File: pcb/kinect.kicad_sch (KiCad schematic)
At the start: 22 parts, among them J2 USB_C_Receptacle_USB2.0_16P, J3 Conn_02x05_Odd_Even, U1 LM3670MFX-1.8, U2 AP63203WU

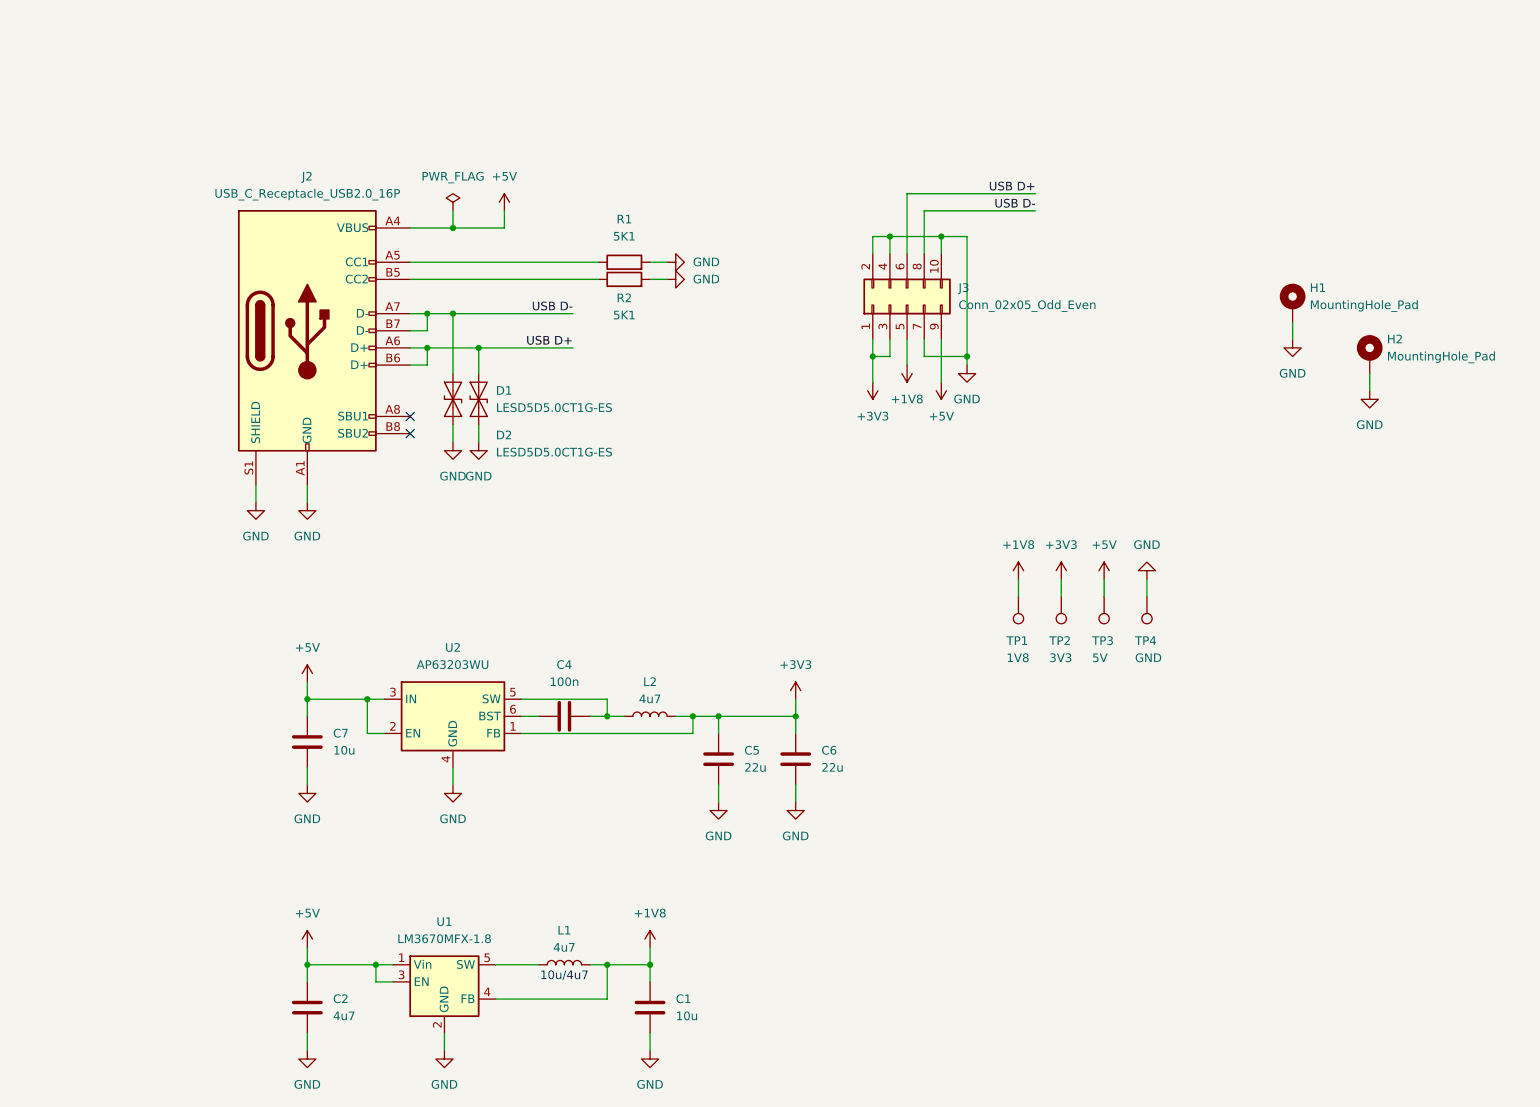
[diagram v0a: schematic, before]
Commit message: Beautified the design.
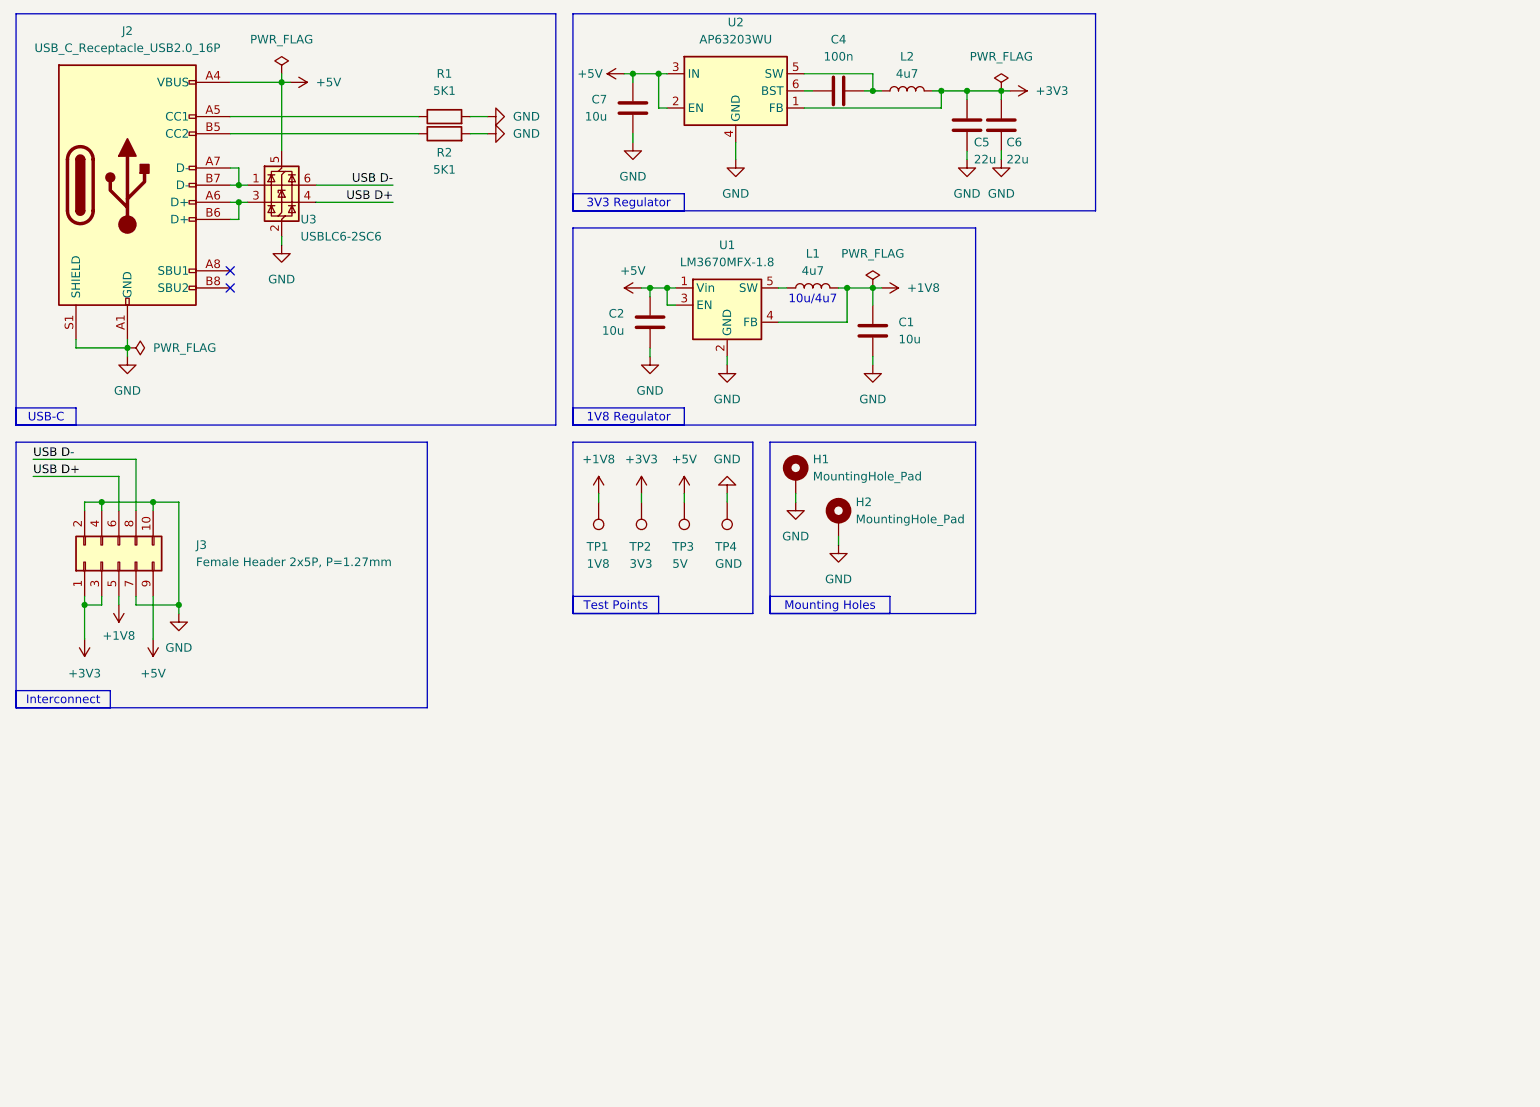
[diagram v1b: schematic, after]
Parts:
- removed D1, D2: LESD5D5.0CT1G-ES, Diode_SMD:D_SOD-523, symbol Diode:SMAJ440CA
- added U3: USBLC6-2SC6, Package_TO_SOT_SMD:SOT-23-6_Handsoldering, symbol Power_Protection:USBLC6-2SC6
- C2: value 4u7 -> 10u; LCSC C2918489 -> C1691
- C4: LCSC (none) -> C6119867
- J3: value Conn_02x05_Odd_Even -> Female Header 2x5P, P=1.27mm
- TP1, TP2, TP3, TP4: now left out of the parts list
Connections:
- net +5V: now also U3.5 (VBUS)
- net GND: now also U3.2 (GND)
- net USB D+: now also U3.4 (I/O2); no longer J2.A6 (D+), J2.B6 (D+)
- net USB D-: now also U3.6 (I/O1); no longer J2.A7 (D-), J2.B7 (D-)
- new net: J2.A7 (D-), J2.B7 (D-), U3.1 (I/O1)
- new net: J2.A6 (D+), J2.B6 (D+), U3.3 (I/O2)
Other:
- moved on the sheet: C1, C4, C5, C6, C7, H1, H2, J2, J3, L1, L2, R1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
